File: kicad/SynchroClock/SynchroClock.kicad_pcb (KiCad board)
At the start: 2 copper layers, 76.2 x 50.8 mm, 30 parts, among them J1 5v IN, J2 serial0, J3 1.5v battery, J4 serial1, J5 ICSP, J6 CLOCK, M1 DS3231-M, SW1 FactoryReset, U1 LM1117-3.3, U2 ESP-12E, U4 DRV8838, U5 ATMEGA328-PU, Y1 8Mhz

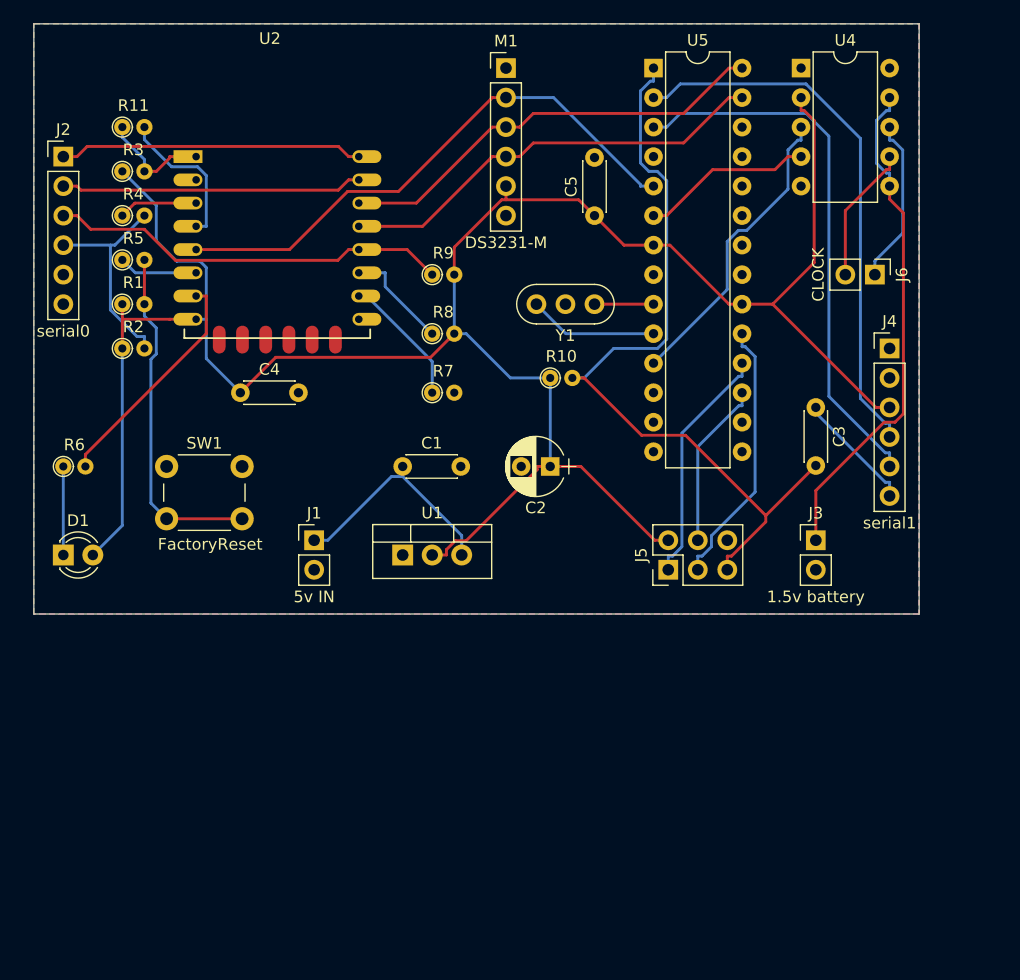
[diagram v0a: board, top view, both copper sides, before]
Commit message: updated hardware design
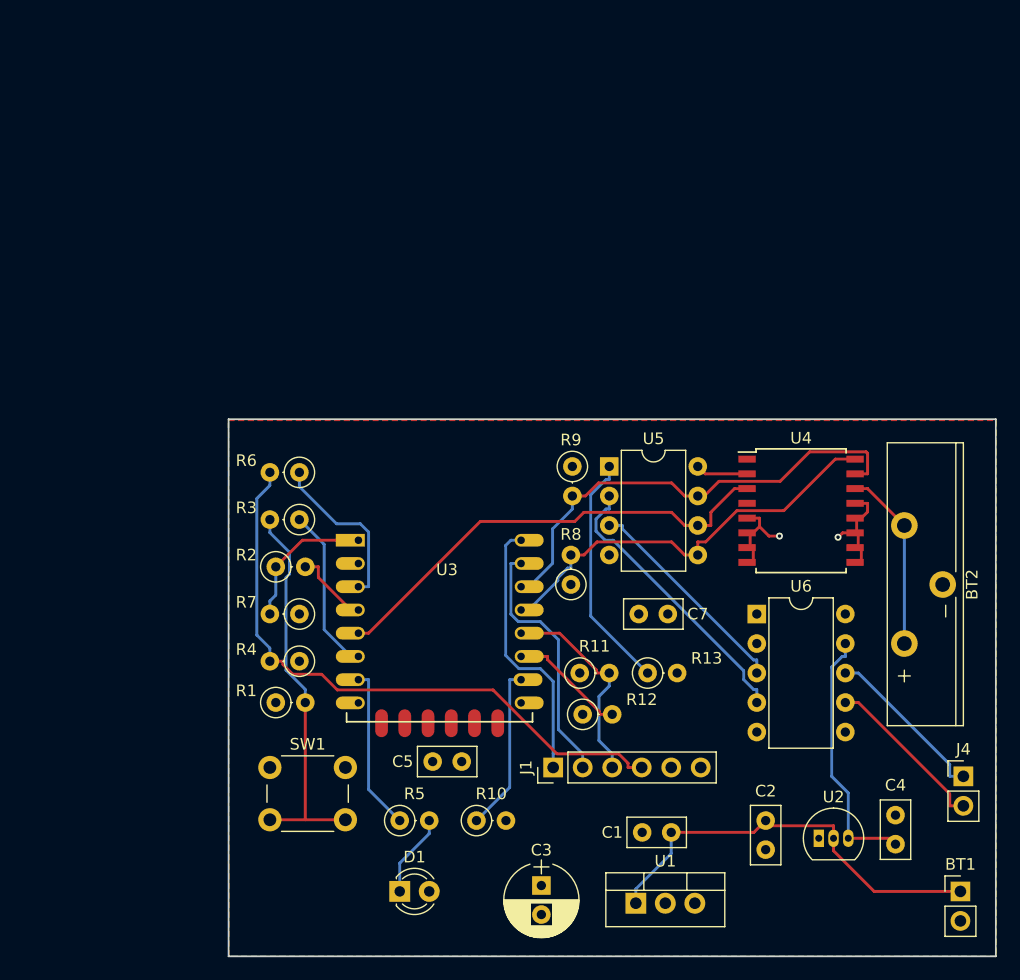
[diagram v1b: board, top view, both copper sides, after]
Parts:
- removed J2: serial0, Pin_Headers:Pin_Header_Straight_1x06_Pitch2.54mm
- removed J3: 1.5v battery, Pin_Headers:Pin_Header_Straight_1x02_Pitch2.54mm
- removed J5: ICSP, Pin_Headers:Pin_Header_Straight_2x03_Pitch2.54mm
- removed J6: CLOCK, Pin_Headers:Pin_Header_Straight_1x02_Pitch2.54mm
- removed M1: DS3231-M, Pin_Headers:Pin_Header_Straight_1x06_Pitch2.54mm
- removed Y1: 8Mhz, Crystals:Resonator_muRata_CSTLSxxxG-3pin_w8.0mm_h3.0mm
- added BT1: 4xAA, Pin_Headers:Pin_Header_Straight_1x02_Pitch2.54mm, F.Cu at (178.8, 122.9)
- added BT2: CR2032, Connectors:CR2032V, F.Cu at (174.0, 91.4)
- added C7: 0.1uf, Capacitors_THT:C_Disc_D5.0mm_W2.5mm_P2.50mm, F.Cu at (151.1, 99.1)
- added R12: 10k, Resistors_THT:R_Axial_DIN0207_L6.3mm_D2.5mm_P2.54mm_Vertical, F.Cu at (146.3, 107.7)
- added R13: 10k, Resistors_THT:R_Axial_DIN0207_L6.3mm_D2.5mm_P2.54mm_Vertical, F.Cu at (151.9, 104.1)
- added U3: ESP-12E, ESP8266:ESP-12E, F.Cu at (127.0, 92.7)
- added U6: DRV8838, Housings_DIP:DIP-10_W7.62mm, F.Cu at (161.3, 99.1)
- C1: value 100nf -> 0.1uf; footprint Capacitors_THT:C_Disc_D4.3mm_W1.9mm_P5.00mm -> Capacitors_THT:C_Disc_D5.0mm_W2.5mm_P2.50mm
- C2: value 100uf -> 0.1uf; footprint Capacitors_THT:CP_Radial_D5.0mm_P2.50mm -> Capacitors_THT:C_Disc_D5.0mm_W2.5mm_P2.50mm
- C3: value 0.1uf -> 100uf; footprint Capacitors_THT:C_Disc_D4.3mm_W1.9mm_P5.00mm -> Capacitors_THT:CP_Radial_D6.3mm_P2.50mm
- C4: value 0.1uf -> 1uf; footprint Capacitors_THT:C_Disc_D4.3mm_W1.9mm_P5.00mm -> Capacitors_THT:C_Disc_D5.0mm_W2.5mm_P2.50mm
- C5: footprint Capacitors_THT:C_Disc_D4.3mm_W1.9mm_P5.00mm -> Capacitors_THT:C_Disc_D5.0mm_W2.5mm_P2.50mm
- J1: value 5v IN -> SERIAL0; footprint Pin_Headers:Pin_Header_Straight_1x02_Pitch2.54mm -> Pin_Headers:Pin_Header_Straight_1x06_Pitch2.54mm
- J4: value serial1 -> CLOCK; footprint Pin_Headers:Pin_Header_Straight_1x06_Pitch2.54mm -> Pin_Headers:Pin_Header_Straight_1x02_Pitch2.54mm
- R1, R10, R7, R8, R9: footprint Resistors_THT:R_Axial_DIN0204_L3.6mm_D1.6mm_P1.90mm_Vertical -> Resistors_THT:R_Axial_DIN0207_L6.3mm_D2.5mm_P2.54mm_Vertical
- R11, R4: value 1k -> 10k; footprint Resistors_THT:R_Axial_DIN0204_L3.6mm_D1.6mm_P1.90mm_Vertical -> Resistors_THT:R_Axial_DIN0207_L6.3mm_D2.5mm_P2.54mm_Vertical
- R2, R3: value 10k -> 1k; footprint Resistors_THT:R_Axial_DIN0204_L3.6mm_D1.6mm_P1.90mm_Vertical -> Resistors_THT:R_Axial_DIN0207_L6.3mm_D2.5mm_P2.54mm_Vertical
- R5: value 1k -> 220; footprint Resistors_THT:R_Axial_DIN0204_L3.6mm_D1.6mm_P1.90mm_Vertical -> Resistors_THT:R_Axial_DIN0207_L6.3mm_D2.5mm_P2.54mm_Vertical
- R6: value 220 -> 1k; footprint Resistors_THT:R_Axial_DIN0204_L3.6mm_D1.6mm_P1.90mm_Vertical -> Resistors_THT:R_Axial_DIN0207_L6.3mm_D2.5mm_P2.54mm_Vertical
- SW1: value FactoryReset -> SW_Push
- U1: value LM1117-3.3 -> TC1262-33VAB
- U2: value ESP-12E -> MCP1702-1502E/TO; footprint ESP8266:ESP-12E -> TO_SOT_Packages_THT:TO-92_Inline_Narrow_Oval
- U4: value DRV8838 -> DS3231; footprint Housings_DIP:DIP-10_W7.62mm -> Housings_SOIC:SOIC-16W_7.5x10.3mm_Pitch1.27mm
- U5: value ATMEGA328-PU -> ATTINY85-20PU; footprint Housings_DIP:DIP-28_W7.62mm -> Housings_DIP:DIP-8_W7.62mm
- moved U2 79.5 mm to (166.6, 118.4)
- moved C4 68.5 mm to (173.2, 118.9), turned to 90 degrees
- moved R11 61.3 mm to (146.1, 104.1)
- moved R5 53.8 mm to (130.6, 116.8)
- moved C5 48.4 mm to (135.9, 111.8), turned to 180 degrees
- moved C3 47.4 mm to (142.7, 122.4)
- moved R4 41.3 mm to (121.9, 103.1), turned to 180 degrees
- moved D1 40.9 mm to (130.6, 122.9)
- moved C1 39.1 mm to (153.9, 117.9), turned to 180 degrees
- moved R10 38.6 mm to (137.2, 116.8)
- moved U4 38.1 mm to (165.1, 90.2)
- moved J4 37.4 mm to (179.1, 113.0)
- moved R1 36.7 mm to (119.9, 106.7)
- moved U1 36.1 mm to (150.9, 124.0)
- moved C2 35.7 mm to (162.1, 116.8), turned to 270 degrees
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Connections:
- C1 pad 1: Net-(C1-Pad1) -> Net-(BT1-Pad1)
- C1 pad 2: GND -> GNDREF
- C2 pad 1: +3.3 -> Net-(BT1-Pad1)
- C2 pad 2: GND -> GNDREF
- C3 pad 1: Net-(C3-Pad1) -> +3V3
- C3 pad 2: /RST1 -> GNDREF
- C4 pad 1: +3.3 -> +1V5
- C4 pad 2: GND -> GNDREF
- C5 pad 1: +3.3 -> GNDREF
- C5 pad 2: GND -> +3V3
- D1 pad 2: +3.3 -> +3V3
- J1 pad 1: Net-(C1-Pad1) -> /TX0
- J1 pad 2: GND -> /RX0
- J4 pad 1: GND -> Net-(J4-Pad1)
- J4 pad 2: GND -> Net-(J4-Pad2)
- R1 pad 1: +3.3 -> +3V3
- R10 pad 1: +3.3 -> Net-(R10-Pad1)
- R10 pad 2: /RST1 -> GNDREF
- R11 pad 1: Net-(R11-Pad1) -> +3V3
- R11 pad 2: Net-(R11-Pad2) -> /GPIO0
- R2 pad 1: +3.3 -> Net-(R2-Pad1)
- R2 pad 2: /RST0 -> Net-(R2-Pad2)
- R3 pad 1: +3.3 -> Net-(R3-Pad1)
- R3 pad 2: Net-(R11-Pad1) -> Net-(R1-Pad2)
- R4 pad 1: Net-(R4-Pad1) -> +3V3
- R5 pad 2: Net-(R1-Pad2) -> Net-(D1-Pad1)
- R6 pad 1: Net-(D1-Pad1) -> Net-(R6-Pad1)
- R6 pad 2: Net-(R6-Pad2) -> /RST0
- R7 pad 1: Net-(R7-Pad1) -> +3V3
- R7 pad 2: GND -> Net-(R2-Pad1)
- R8 pad 1: Net-(R8-Pad1) -> +3V3
- R8 pad 2: +3.3 -> /SDA
- R9 pad 1: /GPIO0 -> +3V3
- R9 pad 2: +3.3 -> /SCL
- SW1 pad 1: GND -> GNDREF
- U1 pad 1: GND -> Net-(BT1-Pad1)
- U1 pad 2: +3.3 -> GNDREF
- U1 pad 3: Net-(C1-Pad1) -> +3V3
- U2 pad 1: Net-(R11-Pad1) -> GNDREF
- U2 pad 2: (no net) -> Net-(BT1-Pad1)
- U2 pad 3: Net-(R4-Pad1) -> +1V5
- U4 pad 1: GND -> (no net)
- U4 pad 10: GND -> GNDREF
- U4 pad 2: +3.3 -> +3V3
- U4 pad 3: Net-(U4-Pad3) -> /1HZ
- U4 pad 4: Net-(U4-Pad4) -> (no net)
- U4 pad 5: (no net) -> GNDREF
- U4 pad 6: +1.5 -> GNDREF
- U4 pad 7: Net-(J6-Pad2) -> GNDREF
- U4 pad 8: Net-(J6-Pad1) -> GNDREF
- U4 pad 9: +1.5 -> GNDREF
- U5 pad 1: /RST1 -> Net-(R13-Pad1)
- U5 pad 2: /RX1 -> Net-(U5-Pad2)
- U5 pad 3: /TX1 -> Net-(U5-Pad3)
- U5 pad 4: (no net) -> GNDREF
- U5 pad 5: /1HZ -> /SDA
- U5 pad 6: Net-(U4-Pad4) -> /1HZ
- U5 pad 7: +3.3 -> /SCL
- U5 pad 8: GND -> +3V3
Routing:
- net +3.3: track 193.9 -> 0.00 mm
- net /RST1: track 68.7 -> 0.00 mm
- net /RX1: track 47.2 -> 0.00 mm
- net /TX1: track 47.2 -> 0.00 mm
- net +1.5: track 43.5 -> 0.00 mm
- net Net-(BT1-Pad1): track 0.00 -> 36.5 mm
- net /RST0: track 18.5 -> 53.4 mm
- net Net-(U4-Pad3): track 26.2 -> 0.00 mm
- net Net-(U5-Pad2): track 0.00 -> 24.7 mm
- net /SCK: track 23.2 -> 0.00 mm
- net +1V5: track 0.00 -> 22.3 mm
- net /MISO: track 20.8 -> 0.00 mm
- net Net-(R13-Pad1): track 0.00 -> 20.6 mm
- net Net-(R6-Pad2): track 19.9 -> 0.00 mm
- net Net-(C1-Pad1): track 19.6 -> 0.00 mm
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- added copper zone on F.Cu, net +3V3
- added copper zone on B.Cu, net GNDREF
- removed copper zone on B.Cu, net GND
- removed copper zone on F.Cu, net GND
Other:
- board size 76.2 x 50.8 mm -> 66 x 46.2 mm
- rule pad_to_mask_clearance: 0 -> 0.2
